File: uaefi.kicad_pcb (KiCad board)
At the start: 4 copper layers, 100 x 100 mm, 159 parts, among them J1 Conn_02x02_Odd_Even, J10 5569-16A2, J11 Conn_02x02_Odd_Even, J12 Conn_02x02_Odd_Even, J13 Conn_02x02_Odd_Even, J14 Conn_02x02_Odd_Even, J15 Conn_02x02_Odd_Even, J16 Conn_02x02_Odd_Even, J17 Conn_02x02_Odd_Even, J18 Conn_02x02_Odd_Even, J19 Conn_02x02_Odd_Even, J2 5569-20A2, J20 Conn_02x02_Odd_Even, J21 Conn_02x02_Odd_Even, J22 Conn_02x02_Odd_Even, J24 Conn_02x02_Odd_Even, J3 5569-06A2, J4 5569-08A2, J5 5569-18A2, J6 Conn_01x06, J7 Conn_01x05_Male, J8 USB_B_Mini, J9 USB_C, M1 Module-power_12and5V-0.2, M2 Module-knock-0.2, M3 Module-vr-discrete-0.5, M4 Module-vr-max9924-0.1, M5 Module-wbo-0.5, M6 Module:mega-mcu100/0.3, M7 Module-can-0.1, P1 Pad, P15 Pad, P16 Pad, P17 Pad, P18 Pad, P2 Pad, P3 Pad, P4 Pad, P5 Pad, P6 Pad, P7 Pad, P8 Pad, Q10 ISL9V3040D3ST, Q11 ISL9V3040D3ST, Q12 ISL9V3040D3ST, Q7 ISL9V3040D3ST, Q8 ISL9V3040D3ST, Q9 ISL9V3040D3ST, U1 TLE9201SG, U10 VNLD5160TR-E, U11 VNLD5160TR-E, U2 TLE9201SG, U3 MPX4/MPXH6400_MAP, U4 MAX31855KASA, U5 JDY-33, U6 VNLD5160TR-E, U7 VNLD5160TR-E, U8 VNLD5160TR-E, U9 VNLD5160TR-E

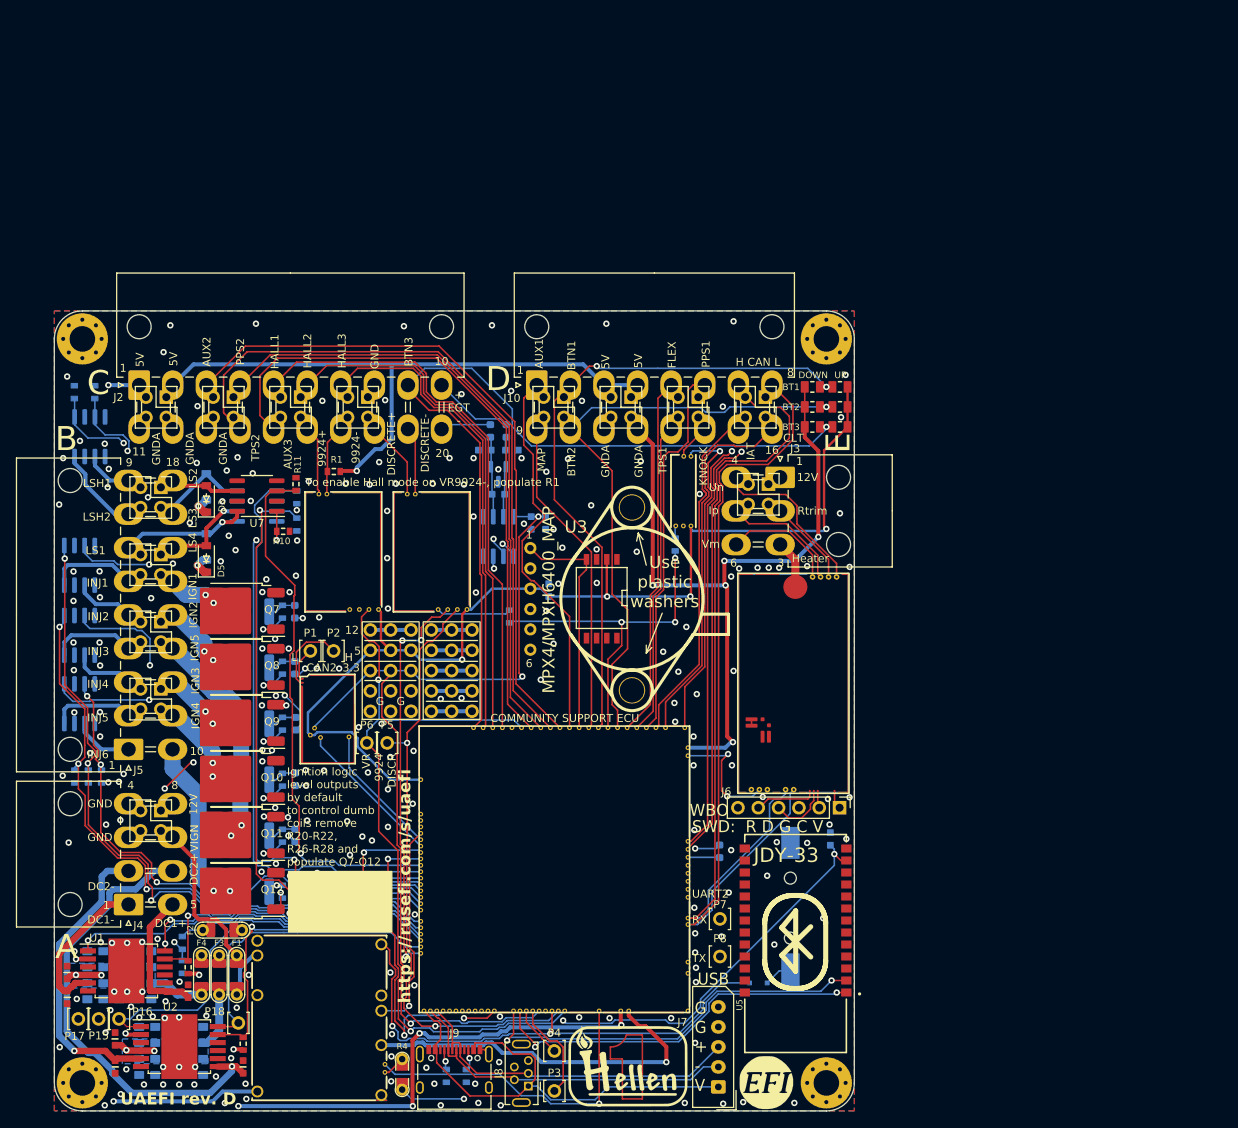
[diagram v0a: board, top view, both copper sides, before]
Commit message: ok
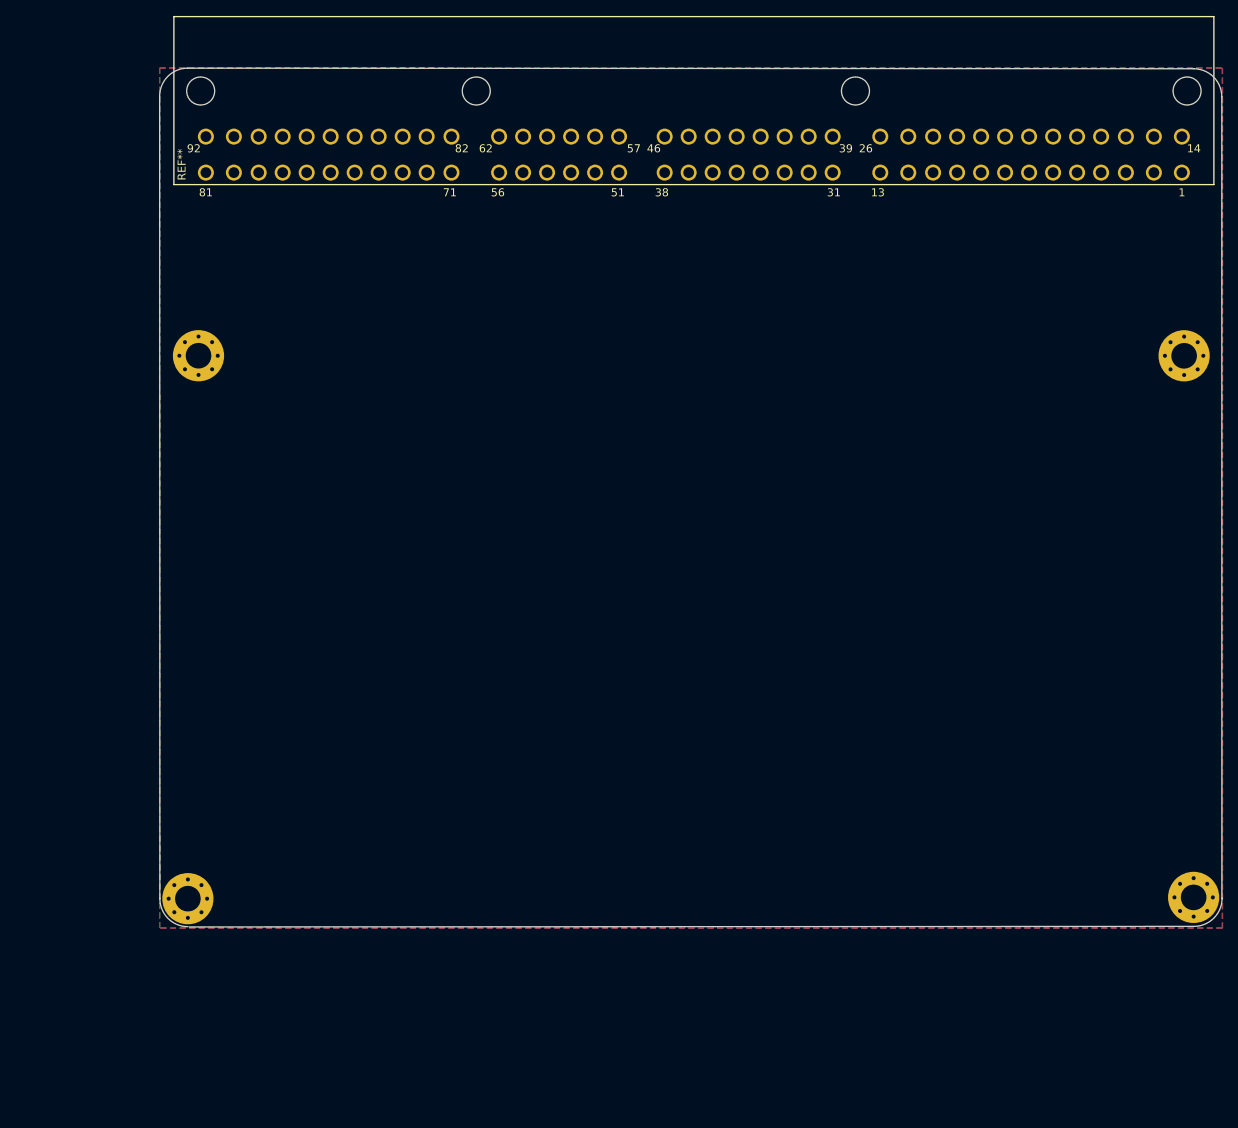
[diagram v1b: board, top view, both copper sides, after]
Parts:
- removed BT1: CR1220, kicad6-libraries:CR1220-2
- removed C1, C10, C14, C15, C16, C17, C18, C19, C2, C20, C21, C22, C23, C3, C4, C5, C6, C7, C8, C9: 10u, hellen-one-common:C0805
- removed C11, C24, C27, C29, C31, C33: 100n, hellen-one-common:C0603
- removed C12, C13, C25, C26, C28, C30: 10n, hellen-one-common:C0603
- removed C32: 1u, hellen-one-common:C0603
- removed D1: 1N4148WS, hellen-one-common:SOD-323
- removed D2, D3, D4, D5: B5819W, hellen-one-common:SOD-123
- removed D8: NUP2105L, Package_TO_SOT_SMD:SOT-23
- removed F1, F2, F3, F4: 12H1500D, hellen-one-common:PAD-1206-PAD
- removed F10, F5, F6, F7, F8, F9: 50mA, Fuse:Fuse_0603_1608Metric
- removed G1: RUSEFI_LOGO, kicad6-libraries:rusefi_logo
- removed G2: LOGO, hellen-one-common:LOGO
- removed G3, G4: PROTO_AREA, hellen-one-common:PROTO_AREA
- removed J1, J11, J12, J13, J14, J15, J16, J17, J18, J19, J20, J21, J22, J24: Conn_02x02_Odd_Even, Connector_PinSocket_2.54mm:PinSocket_2x02_P2.54mm_Vertical
- removed J10: 5569-16A2, Connector_Molex:Molex_Mini-Fit_Jr_5569-16A2_2x08_P4.20mm_Horizontal
- removed J2: 5569-20A2, Connector_Molex:Molex_Mini-Fit_Jr_5569-20A2_2x10_P4.20mm_Horizontal
- removed J3: 5569-06A2, Connector_Molex:Molex_Mini-Fit_Jr_5569-06A2_2x03_P4.20mm_Horizontal
- removed J4: 5569-08A2, Connector_Molex:Molex_Mini-Fit_Jr_5569-08A2_2x04_P4.20mm_Horizontal
- removed J5: 5569-18A2, Connector_Molex:Molex_Mini-Fit_Jr_5569-18A2_2x09_P4.20mm_Horizontal
- removed J6: Conn_01x06, Connector_PinHeader_2.54mm:PinHeader_1x06_P2.54mm_Vertical
- removed J7: Conn_01x05_Male, Connector_Molex:Molex_SPOX_5267-05A_1x05_P2.50mm_Vertical
- removed J8: USB_B_Mini, hellen-one-common:USB-MINI-B-VERTICAL
- removed J9: USB_C, kicad6-libraries:USB_C
- removed L1, L2: 470R@100MHz, Inductor_SMD:L_0603_1608Metric
- removed M1: Module-power_12and5V-0.2, hellen-one-power_12and5V-0.2:power_12and5V
- removed M2: Module-knock-0.2, hellen-one-knock-0.2:knock
- removed M3: Module-vr-discrete-0.5, hellen-one-vr-discrete-0.5:vr-discrete
- removed M4: Module-vr-max9924-0.1, hellen-one-vr-max9924-0.1:vr-max9924
- removed M5: Module-wbo-0.5, hellen-one-wbo-0.5:wbo
- removed M6: Module:mega-mcu100/0.3, hellen-one-mega-mcu100-0.3:mega-mcu100
- removed M7: Module-can-0.1, hellen-one-can-0.1:can
- removed P1, P15, P16, P17, P18, P2, P3, P4, P5, P6, P7, P8: Pad, hellen-one-common:PAD-TH
- removed Q10, Q11, Q12, Q7, Q8, Q9: ISL9V3040D3ST, Package_TO_SOT_SMD:TO-252-2
- removed R1, R10, R11, R12, R13, R14, R15, R16, R29, R30, R31, R32, R33, R34, R9: 4.7k, hellen-one-common:R0603
- removed R17, R18, R19, R23, R24, R25: 22, hellen-one-common:R0603
- removed R2: 33k, hellen-one-common:R0603
- removed R20, R21, R22, R26, R27, R28: 0, Resistor_SMD:R_2512_6332Metric
- removed R3: 6.8k, hellen-one-common:R0603
- removed R35, R36, R37: 10k, hellen-one-common:R0805
- removed R38, R39, R40: DNP, hellen-one-common:R0805
- removed R4: Jumper-Pad-Pad, hellen-one-common:PAD-0805-PAD
- removed R5, R6: 0, hellen-one-common:R0603
- removed R7, R8: 5.6k, hellen-one-common:R0603
- removed U1, U2: TLE9201SG, Package_SO:Infineon_PG-DSO-12-11
- removed U10, U11, U6, U7, U8, U9: VNLD5160TR-E, Package_SO:SOIC-8_3.9x4.9mm_P1.27mm
- removed U3: MPX4/MPXH6400_MAP, kicad6-libraries:MPX-4_MAP
- removed U4: MAX31855KASA, Package_SO:SOIC-8_3.9x4.9mm_P1.27mm
- removed U5: JDY-33, kicad6-libraries:JDY-33
- added REF**: TE-3-178780-6, kicad6-libraries:TE-3-178780-6, F.Cu at (68.9, 38.2)
- moved H3 51.4 mm to (192.4, 133.3)
- moved H4 44.8 mm to (191.2, 65.6)
- moved H2 26.5 mm to (66.7, 133.5)
- moved H1 14.7 mm to (68.0, 65.6)
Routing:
- net +12V_RAW: track 250.7 -> 0.00 mm, vias 2 -> 0
- net +5VP: track 199.7 -> 0.00 mm, vias 3 -> 0
- net +5VA: track 171.8 -> 0.00 mm, vias 6 -> 0
- net +3.3VA: track 169.4 -> 0.00 mm, vias 5 -> 0
- net GNDA: track 155.8 -> 0.00 mm, vias 5 -> 0
- net /LS_HOT1: track 140.6 -> 0.00 mm, vias 2 -> 0
- net /LS_HOT2: track 138.9 -> 0.00 mm, vias 2 -> 0
- net /EGT/SPI_CS: track 111.5 -> 0.00 mm, vias 1 -> 0
- net /IN_BUTTON3: track 109.6 -> 0.00 mm, vias 1 -> 0
- net +3.3V: track 108.0 -> 0.00 mm, vias 8 -> 0
- net /EGT/SPI_SCK: track 107.3 -> 0.00 mm, vias 1 -> 0
- net /EGT/SPI_SO: track 104.7 -> 0.00 mm, vias 1 -> 0
- net /CAN+: track 102.6 -> 0.00 mm
- net /CAN-: track 100.8 -> 0.00 mm
- net /INJ1: track 89.1 -> 0.00 mm, vias 3 -> 0
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- removed copper zone on B.Cu, net /DC Driver 1/PWR
- removed copper zone on B.Cu, net /DC Driver 2/PWR
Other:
- board size 100 x 100 mm -> 132.8 x 107.4 mm
- board text removed: "+ EGT -"
- board text removed: "1"
- board text removed: "10"
- board text removed: "11"
- board text removed: "12"
- board text removed: "12V"
- board text removed: "16"
- board text removed: "18"
- board text removed: "20"
- board text removed: "3"
- board text removed: "3.3"
- board text removed: "4"
- board text removed: "5"
- board text removed: "5V"
- board text removed: "6"
- board text removed: "8"
- board text removed: "9"
- board text removed: "9924+"
- board text removed: "9924-"
- board text removed: "A"
- board text removed: "AUX1"
- board text removed: "AUX2"
- board text removed: "AUX3"
- board text removed: "Always looking for C/C++/PHP/Java developers https://rusefi.com/s/mission"
- board text removed: "B"
- board text removed: "BT1"
- board text removed: "BT2"
- board text removed: "BT3"
- board text removed: "BTN1"
- board text removed: "BTN2"
- board text removed: "BTN3"
- board text removed: "C"
- board text removed: "CAN2"
- board text removed: "CLT"
- board text removed: "COMMUNITY SUPPORT ECU"
- board text removed: "D"
- board text removed: "DC1+"
- board text removed: "DC1-"
- board text removed: "DC2+"
- board text removed: "DC2-"
- board text removed: "DISCRETE+"
- board text removed: "DISCRETE-"
- board text removed: "DOWN"
- board text removed: "E"
- board text removed: "FLEX"
- board text removed: "G"
- board text removed: "G G + - V"
- board text removed: "GND"
- board text removed: "GNDA"
- board text removed: "H"
- board text removed: "H CAN L"
- board text removed: "HALL1"
- board text removed: "HALL2"
- board text removed: "HALL3"
- board text removed: "Heater"
- board text removed: "IAT"
- board text removed: "IGN1"
- board text removed: "IGN2"
- board text removed: "IGN3"
- board text removed: "IGN4"
- board text removed: "IGN5"
- board text removed: "IGN6"
- board text removed: "INJ1"
- board text removed: "INJ2"
- board text removed: "INJ3"
- board text removed: "INJ4"
- board text removed: "INJ5"
- board text removed: "INJ6"
- board text removed: "Ignition logic level outputs by default to control dumb coils remove R20-R22, R26-R28 and populate Q7-Q12"
- board text removed: "Ip"
- board text removed: "KNOCK"
- board text removed: "L"
- board text removed: "L CAN H"
- board text removed: "LS1"
- board text removed: "LS2"
- board text removed: "LS3"
- board text removed: "LS4"
- board text removed: "LSH1"
- board text removed: "LSH2"
- board text removed: "MAP"
- board text removed: "PPS1"
- board text removed: "PPS2"
- board text removed: "Rtrim"
- board text removed: "SWD: R D G C V"
- board text removed: "TPS1"
- board text removed: "TPS2"
- board text removed: "To enable Hall mode on VR9924-, populate R1"
- board text removed: "UAEFI rev. D"
- board text removed: "UART2 RX TX"
- board text removed: "UP"
- board text removed: "USB"
- board text removed: "Un"
- board text removed: "VIGN"
- board text removed: "VR 9924 DISCR"
- board text removed: "Vm"
- board text removed: "WBO"
- board text removed: "https://rusefi.com/s/uaefi"
